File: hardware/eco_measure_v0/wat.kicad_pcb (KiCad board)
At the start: 2 copper layers, 67.2 x 86.2 mm, 48 parts, among them J1 Conn_02x05_Odd_Even, J2 Conn_01x06, J3 Conn_01x03, J4 Conn_01x06, J5 Conn_01x06, P1 V_IN, U1 NANO

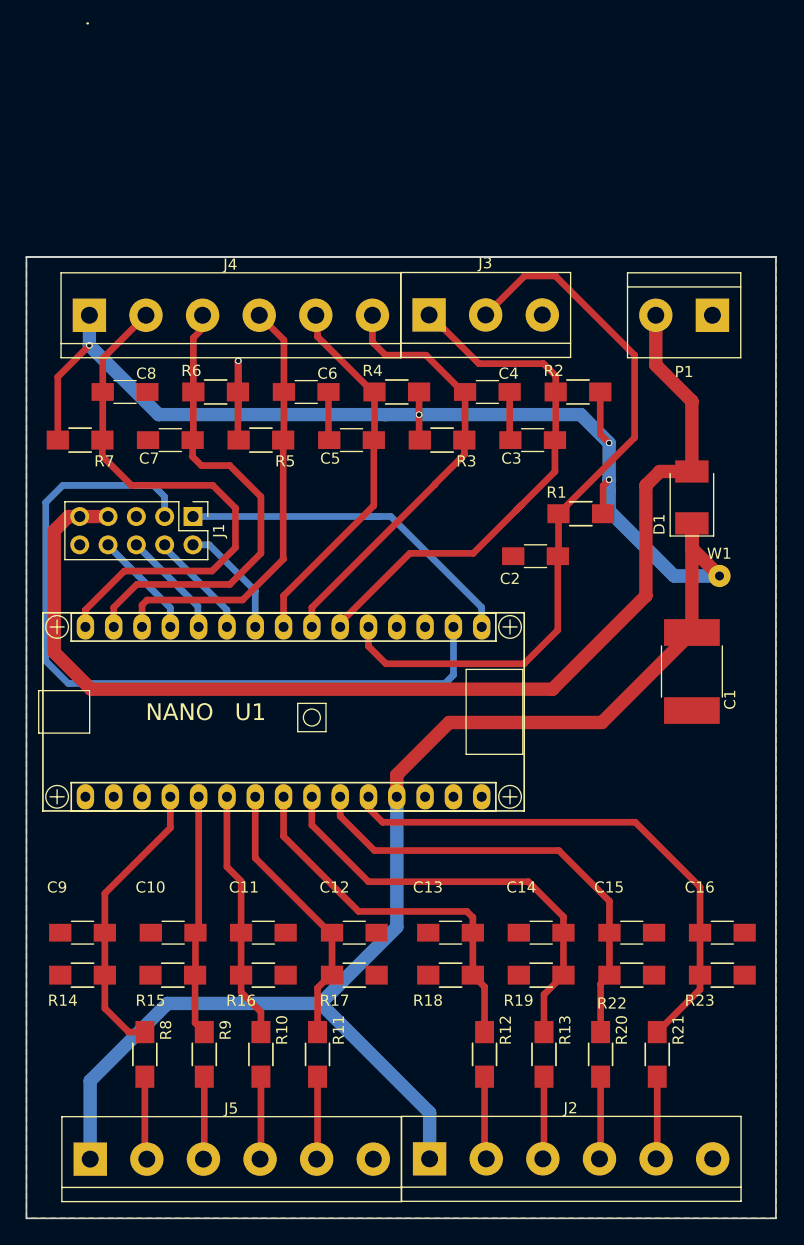
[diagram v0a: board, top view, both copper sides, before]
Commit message: PCB para fabricar
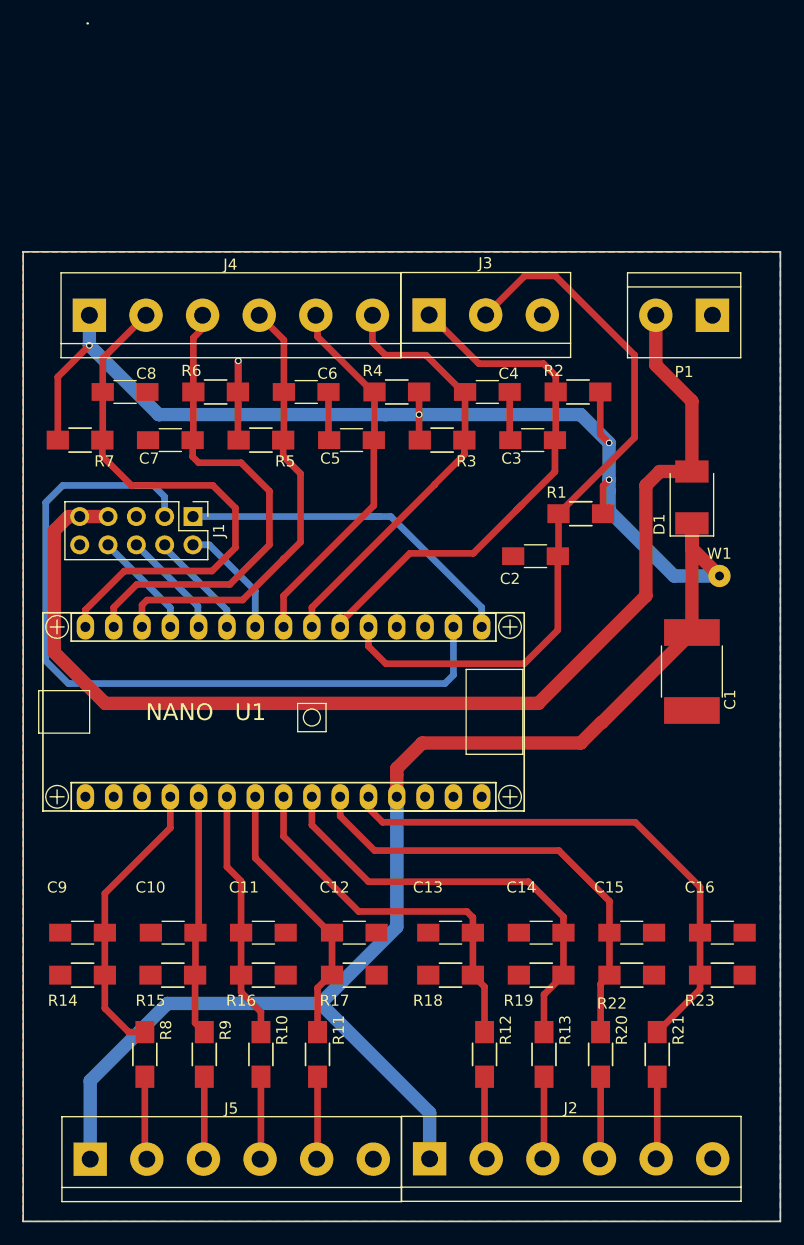
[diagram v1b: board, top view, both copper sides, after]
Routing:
- net /D11: track 42.9 -> 44.3 mm
- net /D10: track 39.2 -> 40.5 mm
- net /vcc_5v: track 104.1 -> 105.2 mm
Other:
- board size 67.2 x 86.2 mm -> 67.9 x 87 mm
